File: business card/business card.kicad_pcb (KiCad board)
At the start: 2 copper layers, 85 x 55 mm, 0 parts

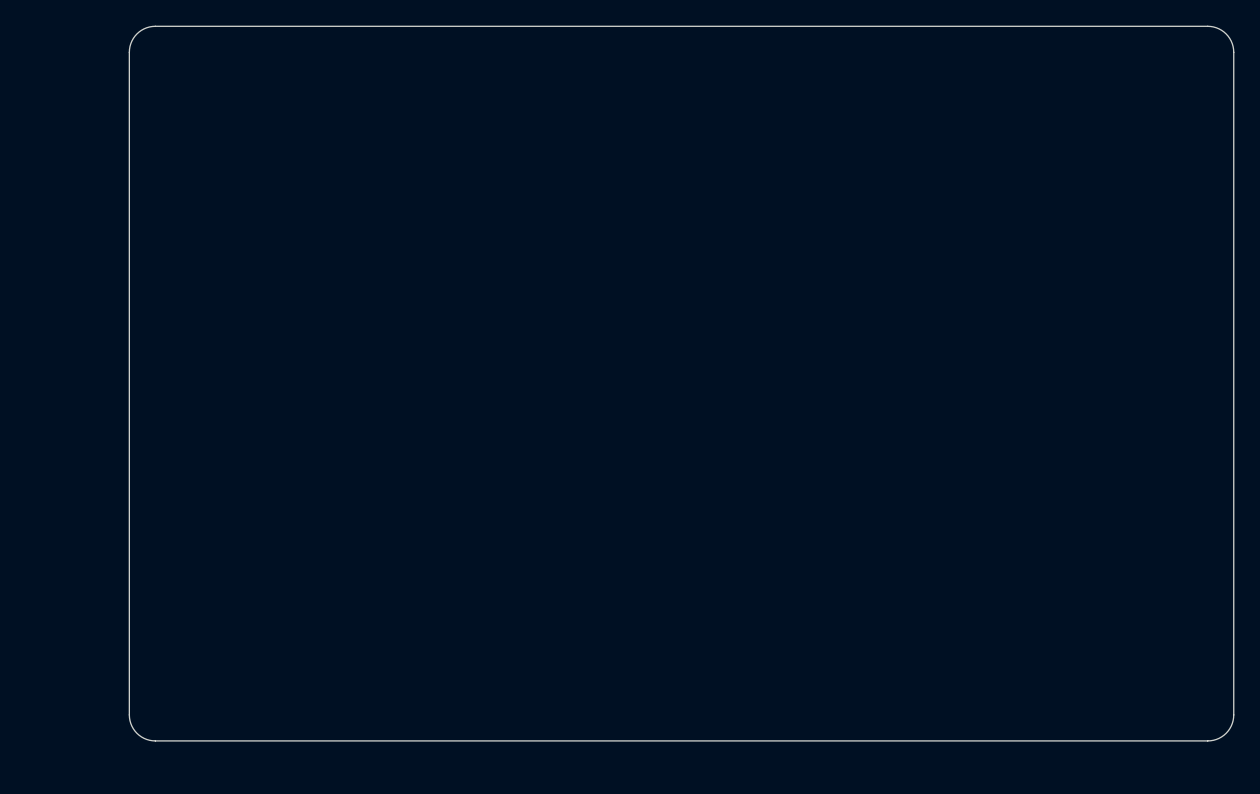
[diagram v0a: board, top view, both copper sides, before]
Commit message: refresh
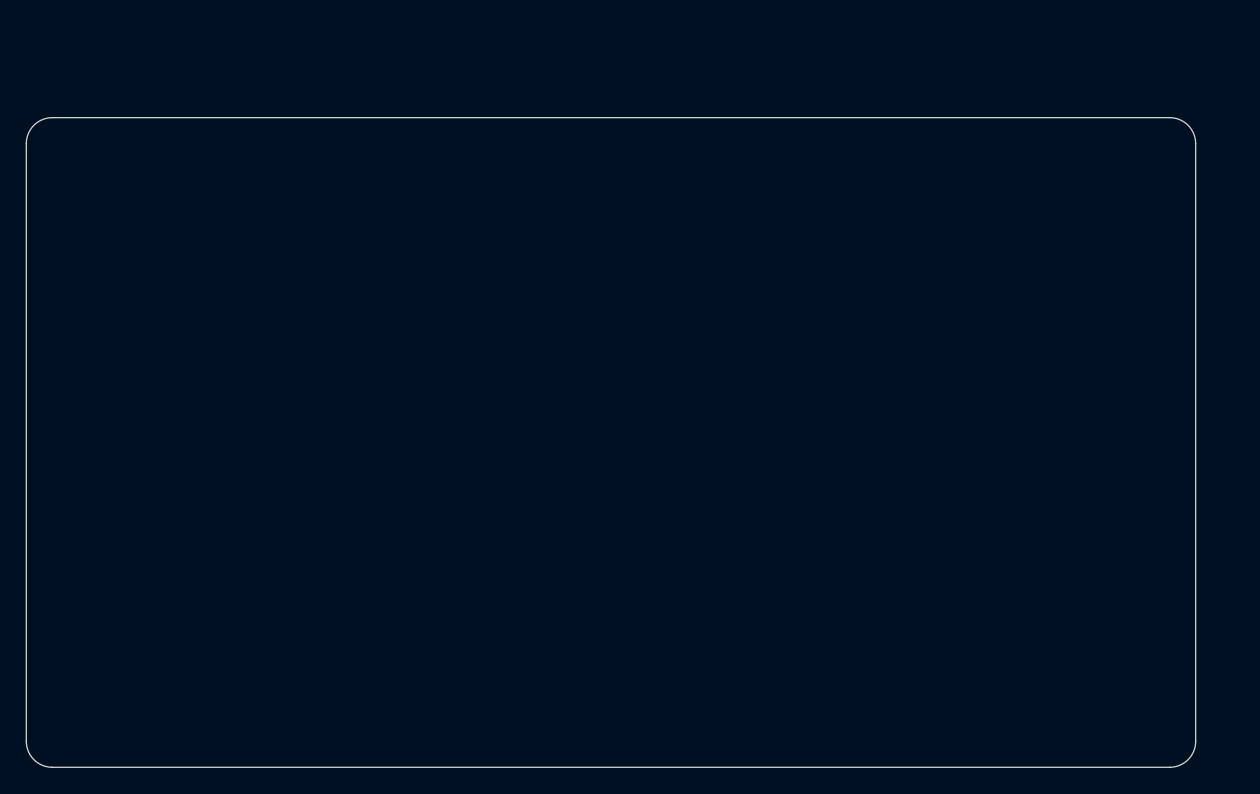
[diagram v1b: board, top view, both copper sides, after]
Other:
- board size 85 x 55 mm -> 90 x 50 mm
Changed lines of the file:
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@@
 	)
 	(gr_arc
-		(start 103.18 75.53)
-		(mid 103.765786 74.115786)
-		(end 105.18 73.53)
+		(start 95.25 82.56)
+		(mid 95.835786 81.145786)
+		(end 97.25 80.56)
 		(stroke
 			(width 0.05)
 			(type default)
 		)
+		(locked yes)
 		(layer "Edge.Cuts")
 	)
 	(gr_line
-		(start 103.18 126.53)
-		(end 103.18 75.53)
+		(start 95.25 128.56)
+		(end 95.25 82.56)
 		(stroke
 			(width 0.05)
 			(type default)
 		)
+		(locked yes)
 		(layer "Edge.Cuts")
 	)
 	(gr_line
-		(start 105.18 73.53)
-		(end 186.18 73.53)
+		(start 97.25 80.56)
+		(end 183.25 80.56)
 		(stroke
 			(width 0.05)
 			(type default)
 		)
+		(locked yes)
 		(layer "Edge.Cuts")
 	)
 	(gr_arc
-		(start 105.18 128.53)
-		(mid 103.765786 127.944214)
-		(end 103.18 126.53)
+		(start 97.25 130.56)
+		(mid 95.835786 129.974214)
+		(end 95.25 128.56)
 		(stroke
 			(width 0.05)
 			(type default)
 		)
+		(locked yes)
 		(layer "Edge.Cuts")
 	)
 	(gr_arc
-		(start 186.18 73.53)
-		(mid 187.594214 74.115786)
-		(end 188.18 75.53)
+		(start 183.25 80.56)
+		(mid 184.664214 81.145786)
+		(end 185.25 82.56)
 		(stroke
 			(width 0.05)
 			(type default)
 		)
+		(locked yes)
 		(layer "Edge.Cuts")
 	)
 	(gr_line
-		(start 186.18 128.53)
-		(end 105.18 128.53)
+		(start 183.25 130.56)
+		(end 97.25 130.56)
 		(stroke
 			(width 0.05)
 			(type default)
 		)
+		(locked yes)
 		(layer "Edge.Cuts")
 	)
 	(gr_line
-		(start 188.18 75.53)
-		(end 188.18 126.53)
+		(start 185.25 82.56)
+		(end 185.25 128.56)
 		(stroke
 			(width 0.05)
 			(type default)
 		)
+		(locked yes)
 		(layer "Edge.Cuts")
 	)
 	(gr_arc
-		(start 188.18 126.53)
-		(mid 187.594214 127.944214)
-		(end 186.18 128.53)
+		(start 185.25 128.56)
+		(mid 184.664214 129.974214)
+		(end 183.25 130.56)
 		(stroke
 			(width 0.05)
 			(type default)
 		)
+		(locked yes)
 		(layer "Edge.Cuts")
 	)
